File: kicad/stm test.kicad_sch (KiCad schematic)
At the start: 2 parts, among them U101 MCP23008-xP

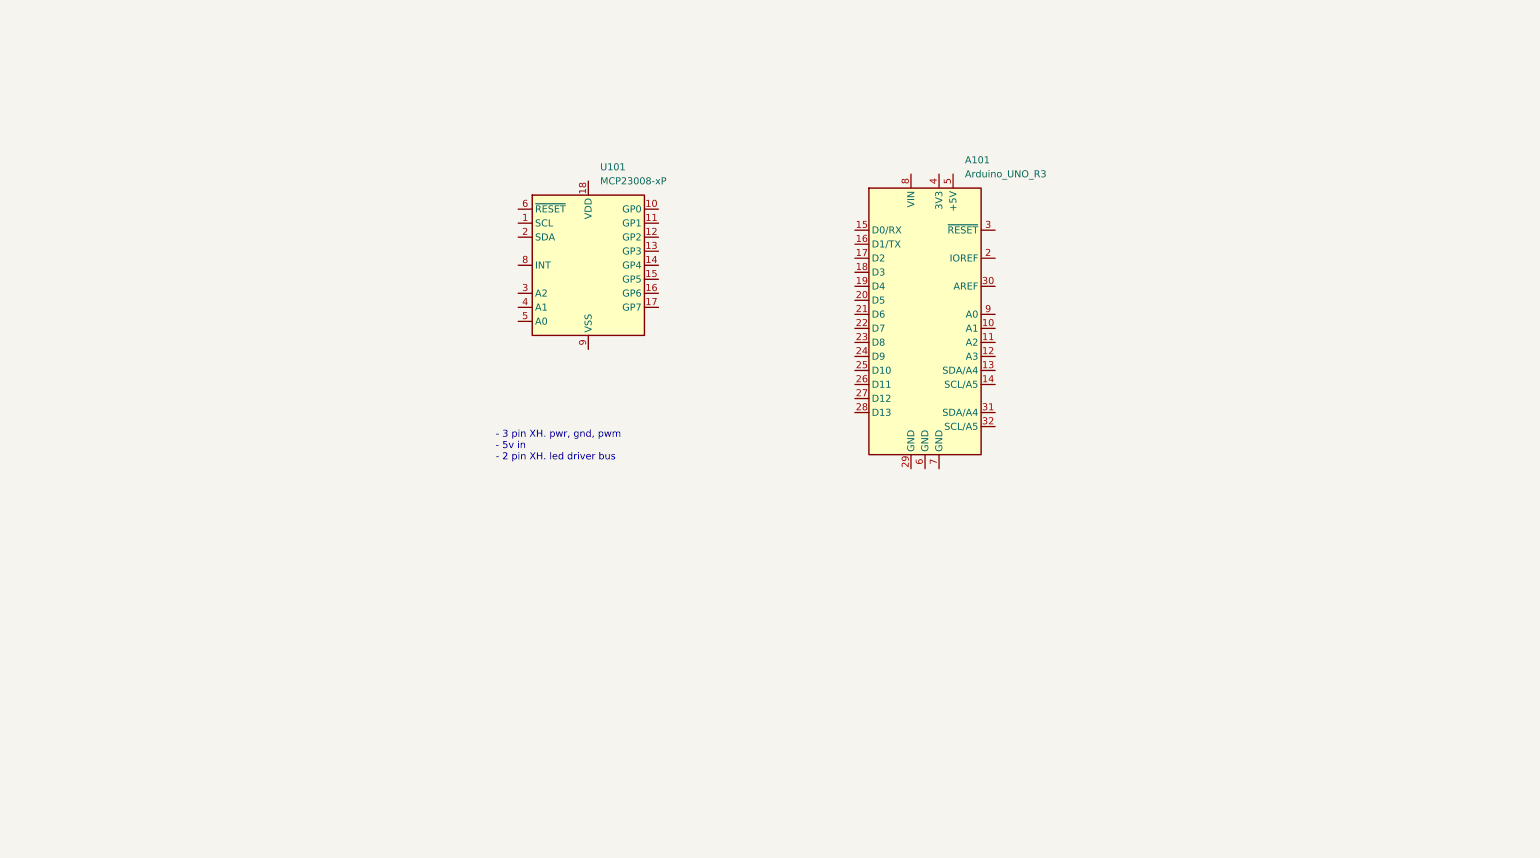
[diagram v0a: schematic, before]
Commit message: womp
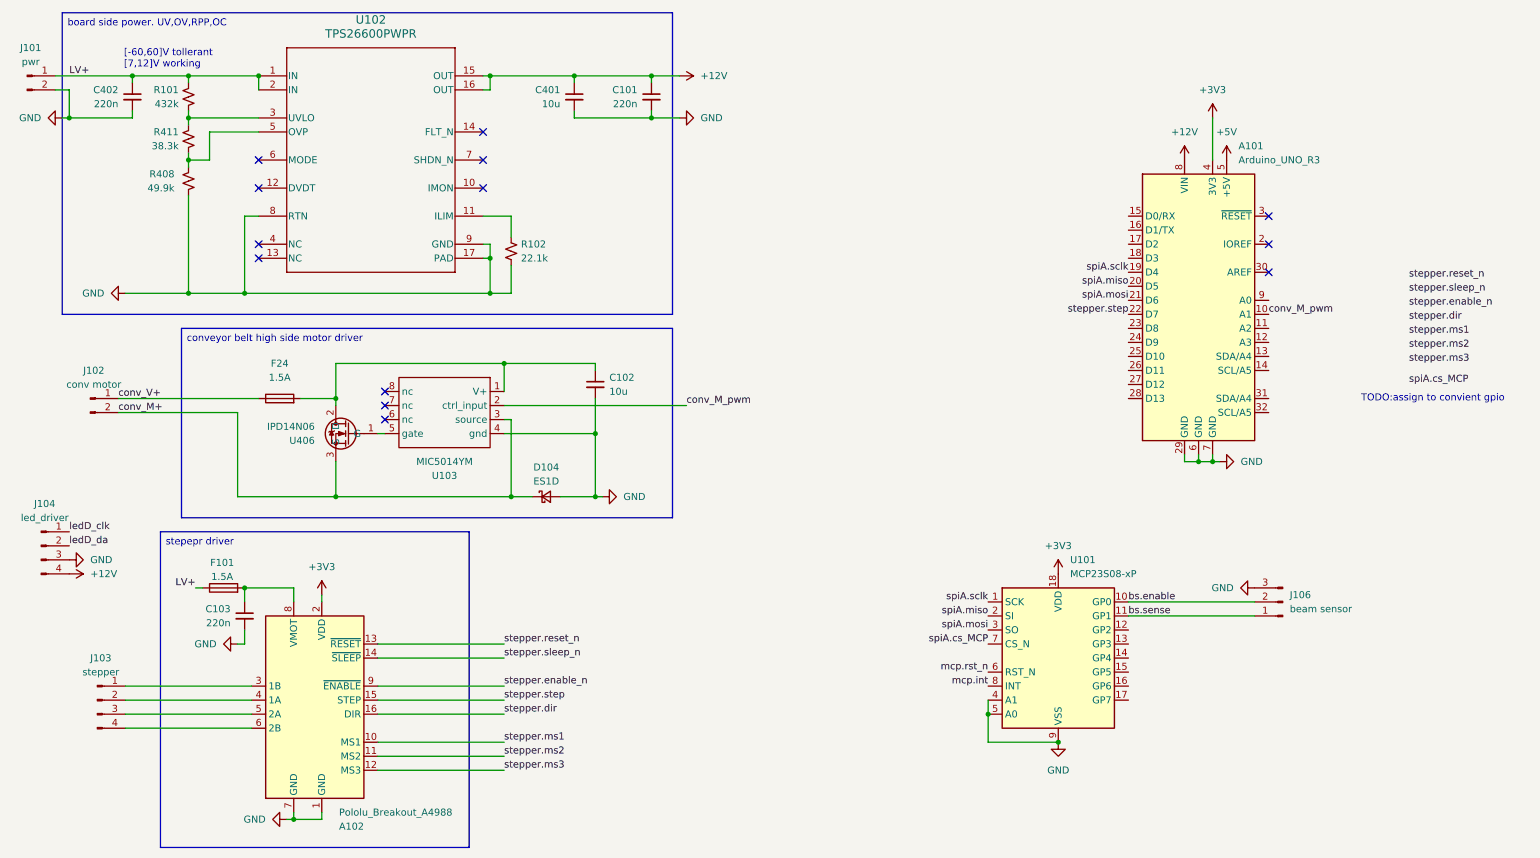
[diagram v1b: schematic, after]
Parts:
- removed U101: MCP23008-xP, Package_DIP:DIP-18_W7.62mm_Socket_LongPads, symbol Interface_Expansion:MCP23008-xP
- added A102: Pololu_Breakout_A4988, Module:Pololu_Breakout-16_15.2x20.3mm, symbol Driver_Motor:Pololu_Breakout_A4988
- added C101, C103, C402: 220n, Capacitor_SMD:C_0805_2012Metric_Pad1.18x1.45mm_HandSolder, symbol Device:C_Small
- added C102, C401: 10u, Capacitor_SMD:C_1206_3216Metric_Pad1.33x1.80mm_HandSolder, symbol Device:C_Small
- added D104: ES1D, Diode_SMD:D_SMA, symbol Device:D_Schottky_Small
- added F101, F24: 1.5A, Resistor_THT:R_Bare_Metal_Element_L21.3mm_W4.8mm_P20.30mm, symbol Device:Fuse
- added J101: pwr, symbol Connector:Conn_01x02_Pin
- added J102: conv motor, TerminalBlock:TerminalBlock_Xinya_XY308-2.54-2P_1x02_P2.54mm_Horizontal, symbol Connector:Conn_01x02_Pin
- added J103: stepper, TerminalBlock:TerminalBlock_Xinya_XY308-2.54-4P_1x04_P2.54mm_Horizontal, symbol Connector:Conn_01x04_Pin
- added J104: led_driver, TerminalBlock:TerminalBlock_Xinya_XY308-2.54-4P_1x04_P2.54mm_Horizontal, symbol Connector:Conn_01x04_Pin
- added J106: beam sensor, TerminalBlock:TerminalBlock_Xinya_XY308-2.54-3P_1x03_P2.54mm_Horizontal, symbol Connector:Conn_01x03_Pin
- added R101: 432k, Resistor_SMD:R_1206_3216Metric_Pad1.30x1.75mm_HandSolder, symbol Device:R_Small_US
- added R102: 22.1k, Resistor_SMD:R_0805_2012Metric_Pad1.20x1.40mm_HandSolder, symbol Device:R_Small_US
- added R408: 49.9k, Resistor_SMD:R_0805_2012Metric_Pad1.20x1.40mm_HandSolder, symbol Device:R_Small_US
- added R411: 38.3k, Resistor_SMD:R_0805_2012Metric_Pad1.20x1.40mm_HandSolder, symbol Device:R_Small_US
- added U101: MCP23S08-xP, Package_DIP:DIP-18_W7.62mm, symbol local:MCP23S08-xP
- added U102: TPS26600PWPR, local:PWP0016H_M, symbol local:TPS26600PWPR
- added U103: MIC5014YM, Package_SO:SOIC-8_3.9x4.9mm_P1.27mm, symbol local:MIC5014
- added U406: IPD14N06, Package_TO_SOT_SMD:TO-252-2, symbol zzLocalLibrary:IPD14N06S2
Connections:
- net conv_M_pwm: now reaches A101.10 (A1)
- net conv_M_pwm: now also U103.2 (ctrl_input)
- net spiA.sclk: now reaches A101.19 (D4)
- net spiA.sclk: now also U101.1 (SCK)
- net spiA.miso: now reaches A101.20 (D5)
- net spiA.miso: now also U101.2 (SI)
- net spiA.mosi: now reaches A101.21 (D6)
- net spiA.mosi: now also U101.3 (SO)
- net stepper.step: now reaches A101.22 (D7)
- net stepper.step: now also A102.15 (STEP)
- net GND: now reaches A101.29 (GND)
- net GND: now also A101.6 (GND), A101.7 (GND), A102.1 (GND), A102.7 (GND), C101.2, C102.2, C103.2, C401.2, C402.2, D104.2 (A), J101.2 (Pin_2), J104.3 (Pin_3), J106.3 (Pin_3), R102.1, R408.1, U101.4 (A1), U101.5 (A0), U101.9 (VSS), U102.17 (PAD), U102.8 (RTN), U102.9 (GND), U103.4 (gnd)
- net +3V3: now reaches A101.4 (3V3)
- net +3V3: now also A102.2 (VDD), U101.18 (VDD)
- net +5V: now reaches A101.5 (+5V)
- net +12V: now reaches A101.8 (VIN)
- net +12V: now also C101.1, C401.1, J104.4 (Pin_4), U102.15 (OUT), U102.16 (OUT)
- new net: A102.3 (1B), J103.1 (Pin_1)
- new net: A102.4 (1A), J103.2 (Pin_2)
- new net: A102.5 (2A), J103.3 (Pin_3)
- new net: A102.6 (2B), J103.4 (Pin_4)
- new net: R102.2, U102.11 (ILIM)
- new net: R408.2, R411.1, U102.5 (OVP)
- new net: A102.8 (VMOT), C103.1, F101.2
- new net: C102.1, F24.2, U103.1 (V+), U406.2 (D)
- new net: R101.1, R411.2, U102.3 (UVLO)
- new net: U103.5 (gate), U406.1 (G)
- new net LV+: C402.1, F101.1, J101.1 (Pin_1), R101.2, U102.1 (IN), U102.2 (IN)
- new net bs.enable: J106.2 (Pin_2), U101.10 (GP0)
- new net bs.sense: J106.1 (Pin_1), U101.11 (GP1)
- new net conv_M+: D104.1 (K), J102.2 (Pin_2), U103.3 (source), U406.3 (S)
- new net conv_V+: F24.1, J102.1 (Pin_1)
- new net ledD_clk: J104.1 (Pin_1)
- new net ledD_da: J104.2 (Pin_2)
- new net mcp.int: U101.8 (INT)
- new net mcp.rst_n: U101.6 (RST_N)
- new net spiA.cs_MCP: U101.7 (CS_N)
- new net stepper.dir: A102.16 (DIR)
- new net stepper.enable_n: A102.9 (~{ENABLE})
- new net stepper.ms1: A102.10 (MS1)
- new net stepper.ms2: A102.11 (MS2)
- new net stepper.ms3: A102.12 (MS3)
- new net stepper.reset_n: A102.13 (~{RESET})
- new net stepper.sleep_n: A102.14 (~{SLEEP})
- no-connect marks 0 -> 13
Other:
- note added: "TODO:assign to convient gpio"
- note added: "[-60,60]V tollerant [7,12]V working"
- note removed: "- 3 pin XH. pwr, gnd, pwm - 5v in - 2 pin XH. led driver bus"
- moved on the sheet: A101
